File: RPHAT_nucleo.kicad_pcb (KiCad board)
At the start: 2 copper layers, 2 parts, among them J1 Raspberry_Pi_2_3, U1 NUCLEO-F446RE

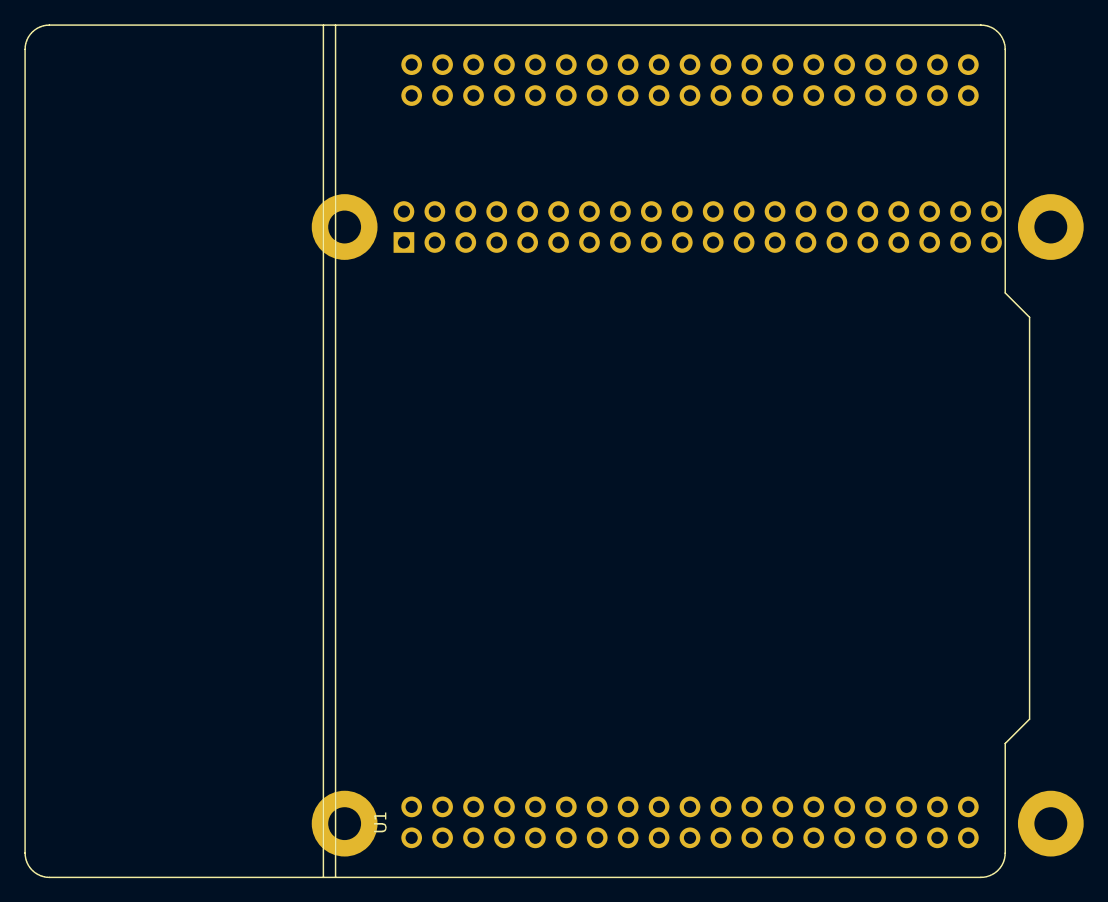
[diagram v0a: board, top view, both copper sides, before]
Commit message: to 6.0
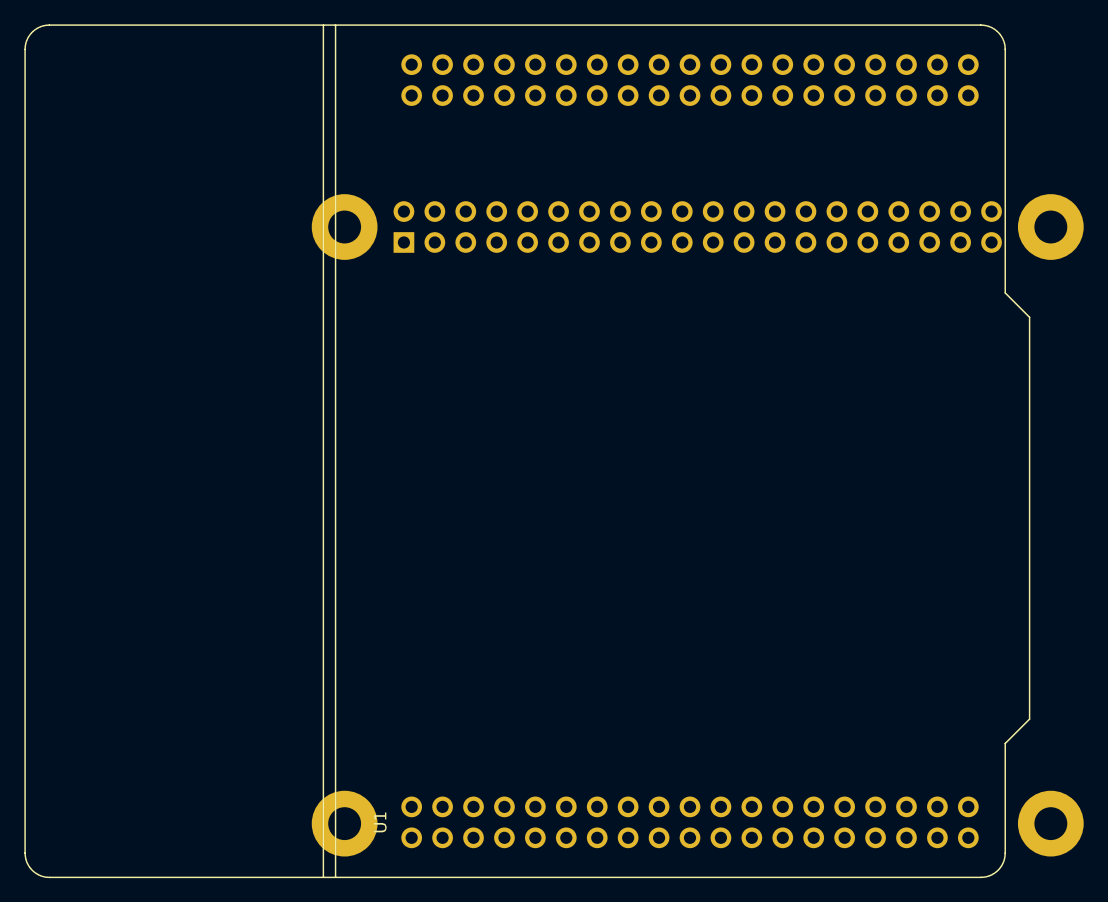
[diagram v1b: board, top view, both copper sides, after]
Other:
- net class Default removed
